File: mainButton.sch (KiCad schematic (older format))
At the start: 34 parts

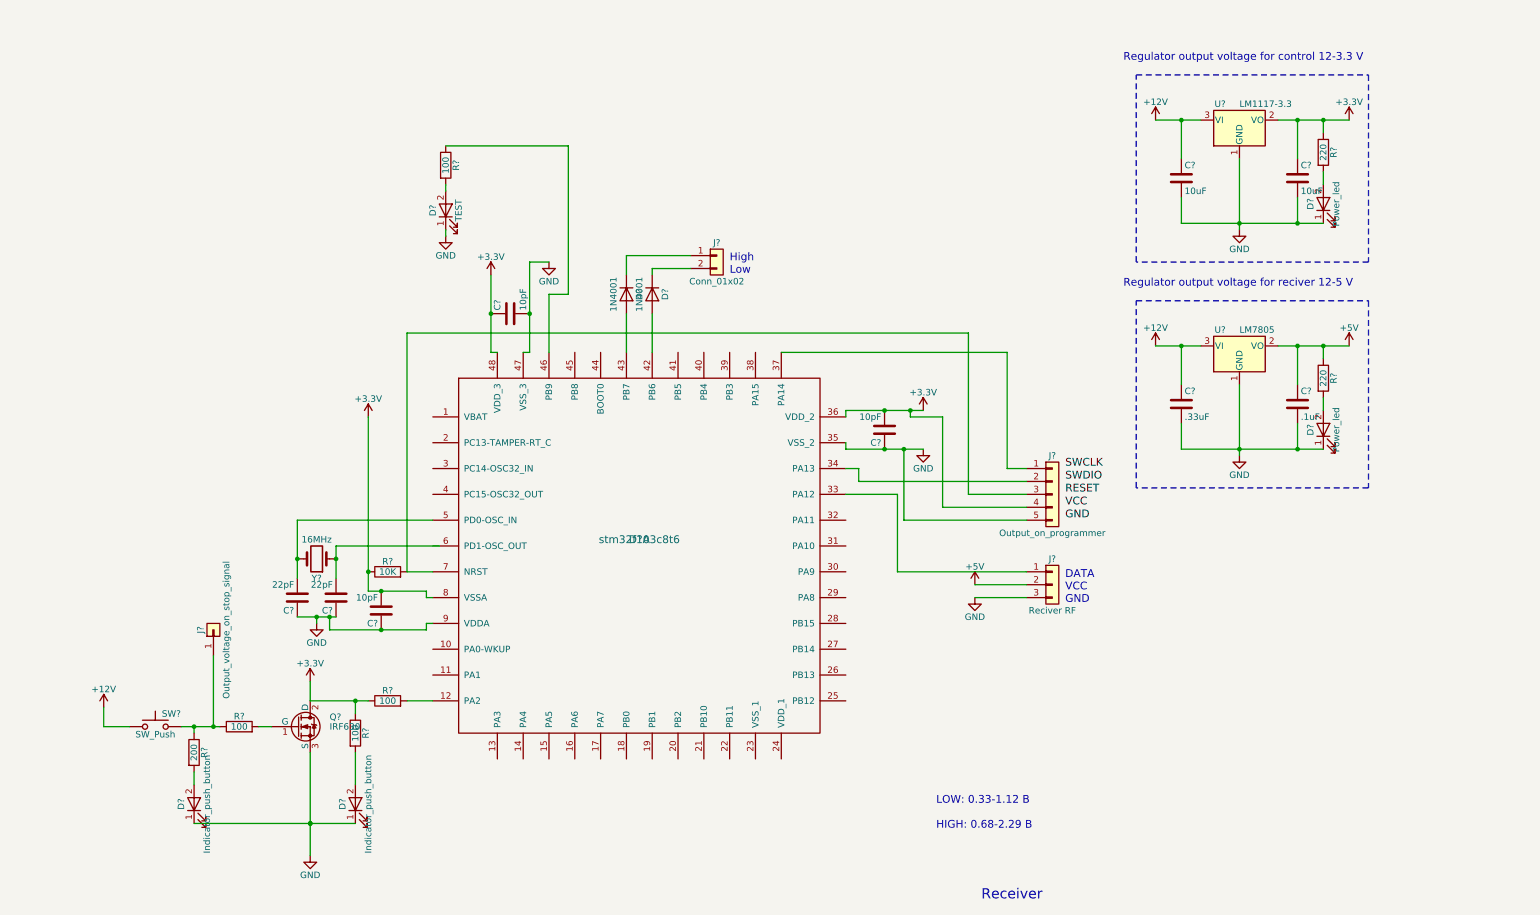
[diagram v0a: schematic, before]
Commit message: Add files via upload
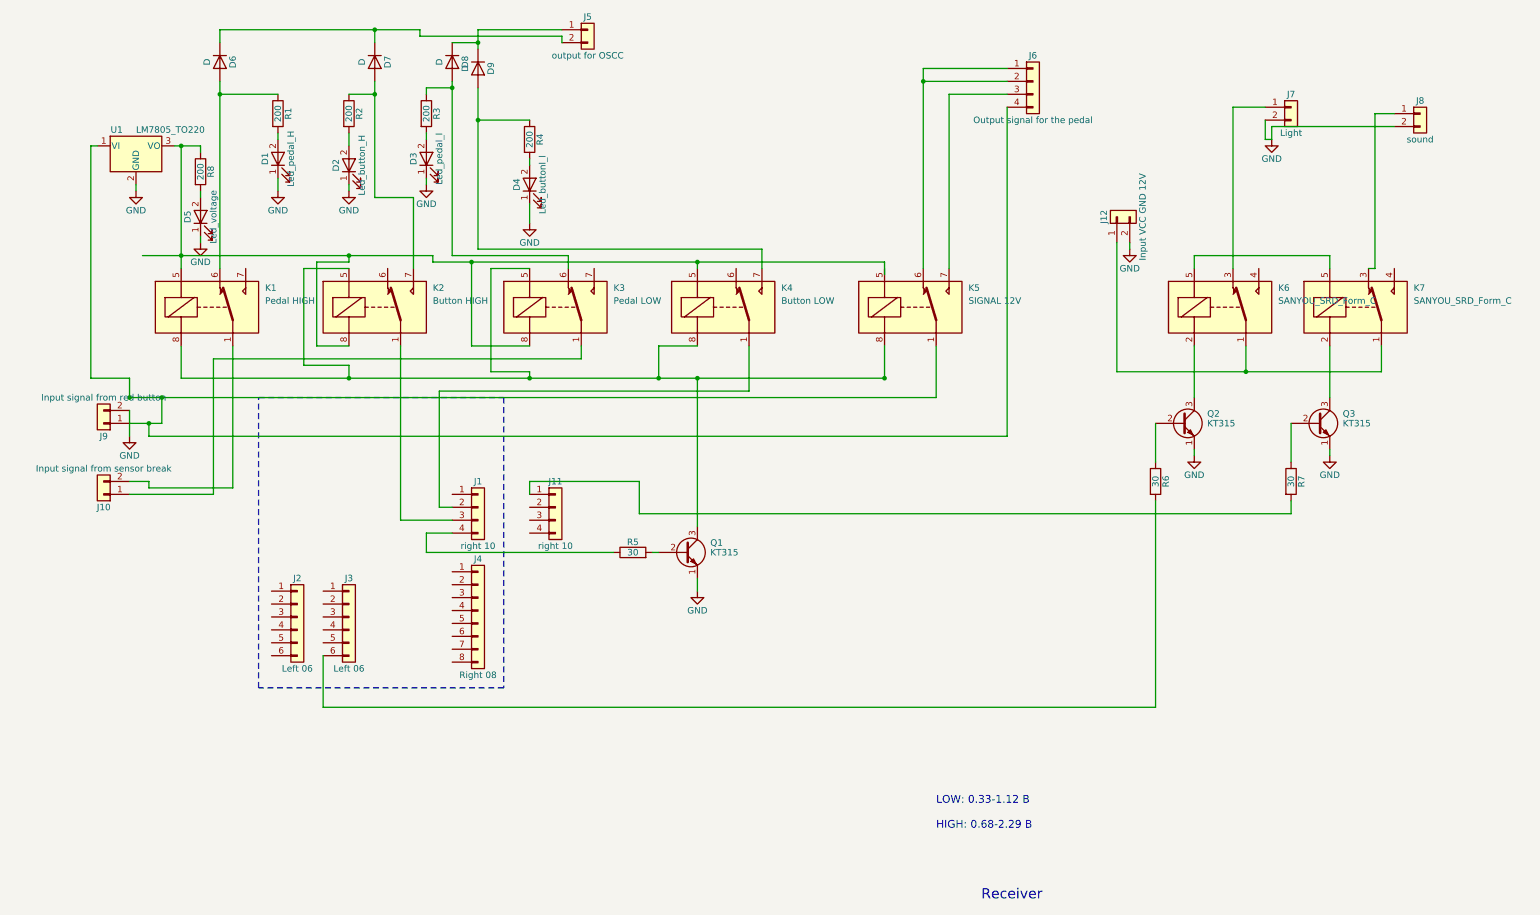
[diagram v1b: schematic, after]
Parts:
- removed C? (x2): 10uF, symbol C
- removed C? (x3): 10pF, symbol C
- removed C? (x2): 22pF, symbol C
- removed C?: .33uF, symbol C
- removed C?: .1uF, symbol C
- removed D? (x2): Power_led, symbol LED
- removed D? (x2): Indicator_push_button, symbol LED
- removed D?: TEST, symbol LED
- removed D? (x2): 1N4001, symbol D
- removed D?: stm32f103c8t6, symbol stm32f103c8t6
- removed J?: Output_on_programmer, symbol Conn_01x05
- removed J?: Conn_01x02, symbol Conn_01x02
- removed J?: Output_voltage_on_stop_signal, symbol Conn_01x01
- removed J?: Reciver RF, symbol Conn_01x03
- removed Q?: IRF630, TO_SOT_Packages_THT:TO-220_Vertical, symbol IRF3205
- removed R?: 10K, symbol R
- removed R? (x2): 220, symbol R
- removed R? (x4): 100, symbol R
- removed R?: 200, symbol R
- removed SW?: SW_Push, symbol SW_Push
- removed U?: LM1117-3.3, symbol LM1117-3.3
- removed U?: LM7805, symbol LM1117-3.3
- removed Y?: 16MHz, symbol Crystal
- added D1: Led_pedal_H, LEDs:LED_D3.0mm, symbol LED
- added D2: Led_button_H, LEDs:LED_D3.0mm, symbol LED
- added D3: Led_pedal_l, LEDs:LED_D3.0mm, symbol LED
- added D4: Led_buttonl_l, LEDs:LED_D3.0mm, symbol LED
- added D5: Led_voltage, LEDs:LED_D5.0mm, symbol LED
- added D6, D7, D8, D9: D, Diodes_THT:D_DO-35_SOD27_P7.62mm_Horizontal, symbol D
- added J1, J11: right 10, Socket_Strips:Socket_Strip_Straight_1x04_Pitch2.54mm, symbol Conn_01x04
- added J10: Input signal from sensor break, Connectors_Phoenix:PhoenixContact_MC-G_02x3.50mm_Angled, symbol Conn_01x02
- added J12: Input VCC GND 12V, Connectors_Phoenix:PhoenixContact_MC-G_02x3.50mm_Angled, symbol Conn_01x02
- added J2, J3: Left 06, Socket_Strips:Socket_Strip_Straight_1x06_Pitch2.54mm, symbol Conn_01x06
- added J4: Right 08, Socket_Strips:Socket_Strip_Straight_1x08_Pitch2.54mm, symbol Conn_01x08
- added J5: output for OSCC, Connectors_Phoenix:PhoenixContact_MC-G_02x3.50mm_Angled, symbol Conn_01x02
- added J6: Output signal for the pedal, Connectors_Phoenix:PhoenixContact_MC-G_04x3.50mm_Angled, symbol Conn_01x04
- added J7: Light, Connectors_JST:JST_NV_B02P-NV_2x5.00mm_Vertical, symbol Conn_01x02
- added J8: sound, Connectors_JST:JST_NV_B02P-NV_2x5.00mm_Vertical, symbol Conn_01x02
- added J9: Input signal from red button, Connectors_Phoenix:PhoenixContact_MC-G_02x3.50mm_Angled, symbol Conn_01x02
- added K1: Pedal HIGH, Relays_THT:Relay_SPDT_HJR-4102, symbol FINDER-40.51-RESCUE-mainButton
- added K2: Button HIGH, Relays_THT:Relay_SPDT_HJR-4102, symbol FINDER-40.51-RESCUE-mainButton
- added K3: Pedal LOW, Relays_THT:Relay_SPDT_HJR-4102, symbol FINDER-40.51-RESCUE-mainButton
- added K4: Button LOW, Relays_THT:Relay_SPDT_HJR-4102, symbol FINDER-40.51-RESCUE-mainButton
- added K5: SIGNAL 12V, Relays_THT:Relay_SPDT_HJR-4102, symbol FINDER-40.51-RESCUE-mainButton
- added K6, K7: SANYOU_SRD_Form_C, Relays_THT:Relay_SPDT_SANYOU_SRD_Series_Form_C, symbol SANYOU_SRD_Form_C
- added Q1, Q2, Q3: KT315, TO_SOT_Packages_THT:TO-92_Inline_Narrow_Oval, symbol 2N2219
- added R1, R2, R3, R4, R8: 200, SMD_Packages:SMD-1206_Pol, symbol R
- added R5, R6, R7: 30, SMD_Packages:SMD-1206_Pol, symbol R
- added U1: LM7805_TO220, TO_SOT_Packages_THT:TO-220-3_Horizontal, symbol LM7805_TO220
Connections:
- net GND: now also D1.1 (K), D2.1 (K), D3.1 (K), D4.1 (K), D5.1 (K), J12.2 (Pin_2), J7.2 (Pin_2), J8.2 (Pin_2), J9.2 (Pin_2), Q1.1 (E), Q2.1 (E), Q3.1 (E), U1.2 (GND)
- new net: J10.2 (Pin_2), K1.1
- new net: K1.5, K2.8, K3.8, K4.5, R8.1, U1.3 (VO)
- new net: D6.2 (A), K1.6, R1.1
- new net: K1.8, K2.5, K3.5, K4.8, K5.8, Q1.3 (C)
- new net: J1.3 (Pin_3), K2.1
- new net: D7.2 (A), K2.7, R2.1
- new net: J10.1 (Pin_1), K3.1
- new net: D8.2 (A), K3.6, R3.1
- new net: J1.2 (Pin_2), K4.1
- new net: D9.2 (A), K4.7, R4.1
- new net: J6.4 (Pin_4), J9.1 (Pin_1), K5.1, U1.1 (VI)
- new net: J6.1 (Pin_1), J6.2 (Pin_2), K5.6
- new net: J6.3 (Pin_3), K5.7
- new net: Q1.2 (B), R5.2
- new net: J1.4 (Pin_4), R5.1
- new net: Q2.2 (B), R6.1
- new net: K6.2, Q2.3 (C)
- new net: Q3.2 (B), R7.1
- new net: K7.2, Q3.3 (C)
- new net: D1.2 (A), R1.2
- new net: D2.2 (A), R2.2
- new net: D3.2 (A), R3.2
- new net: D4.2 (A), R4.2
- new net: J7.1 (Pin_1), K6.3
- new net: J3.6 (Pin_6), R6.2
- new net: J11.1 (Pin_1), R7.2
- new net: J12.1 (Pin_1), K6.1, K7.1
- new net: K6.5, K7.5
- new net: J8.1 (Pin_1), K7.3
- new net: D5.2 (A), R8.2
- new net: D8.1 (K), D9.1 (K), J5.1 (Pin_1)
- new net: D6.1 (K), D7.1 (K), J5.2 (Pin_2)
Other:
- note removed: "DATA\nVCC\nGND"
- note removed: "High\nLow\n"
- note removed: "Regulator output voltage for control 12-3.3 V\n"
- note removed: "Regulator output voltage for reciver 12-5 V\n"
